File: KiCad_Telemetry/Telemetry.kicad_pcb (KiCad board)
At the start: 2 copper layers, 67 x 51 mm, 45 parts, among them IC1 TCAN1044VDRQ1, J2 Conn_01x03, J3 PinHeader_01x02, J4 PinHeader_01x02, J7 DB9_Female, J8 USB Micro Connector, U1 NRF24L01_Breakout, U2 STM32F042C4T6, U3 LD3985M33R_SOT23, U4 MCP2518FDT, Y1 Crystal_GND24

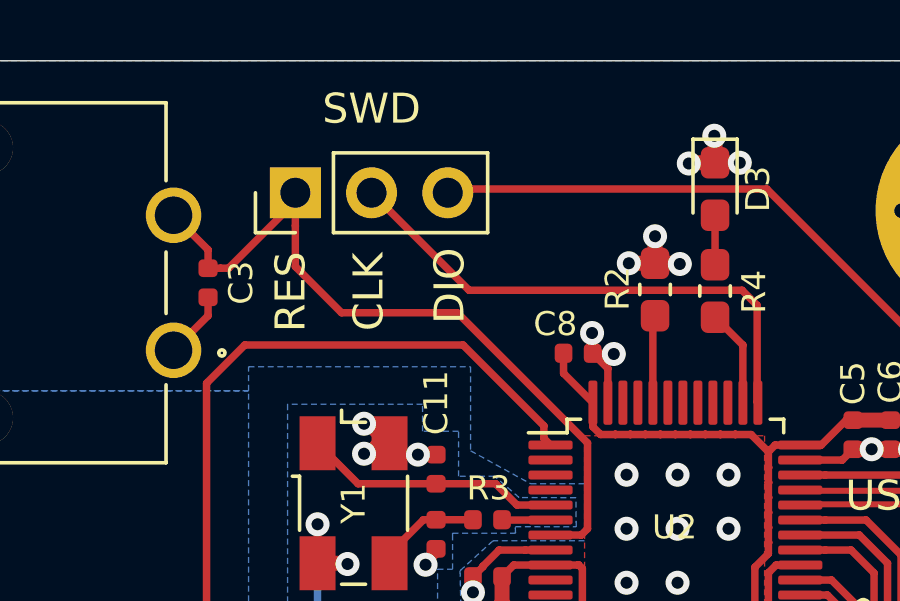
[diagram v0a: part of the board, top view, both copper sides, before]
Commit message: Updated final files for hand-in
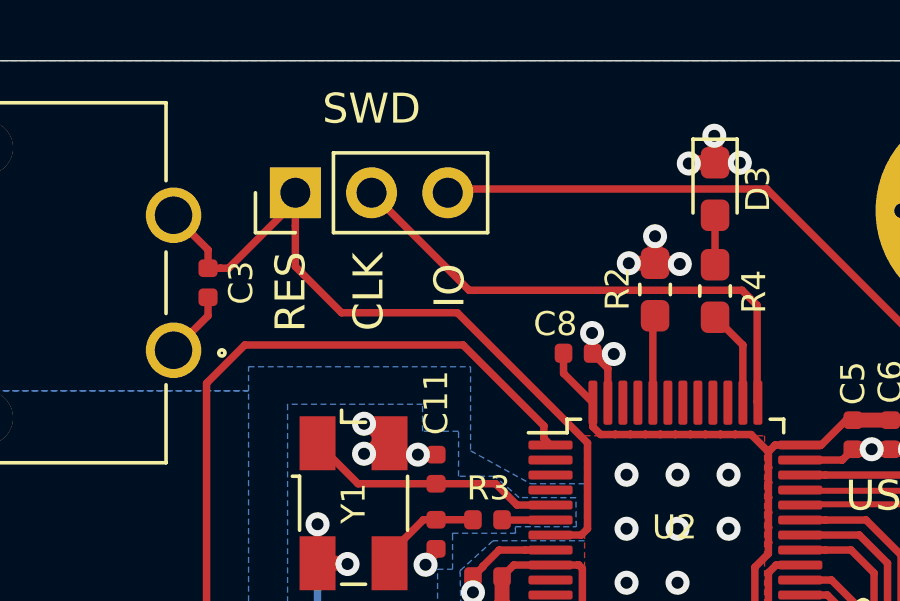
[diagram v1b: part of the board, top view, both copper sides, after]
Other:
- board text added: "IO"
- board text removed: "DIO"
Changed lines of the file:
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@@
     (effects (font (size 1 1) (thickness 0.15)))
   )
-  (gr_text DIO (at 227.3 106.5 90) (layer F.SilkS)
+  (gr_text IO (at 227.3 106.5 90) (layer F.SilkS)
     (effects (font (size 1 1) (thickness 0.15)))
   )
